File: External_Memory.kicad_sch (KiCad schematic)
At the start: 2 parts, among them U5 GD25D10CT

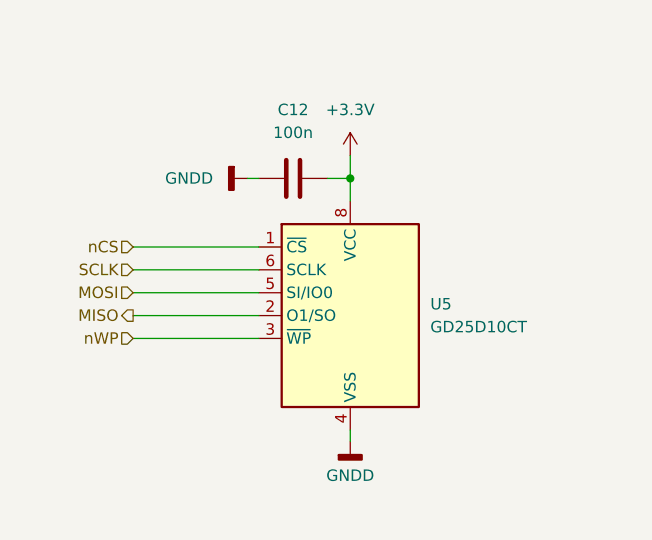
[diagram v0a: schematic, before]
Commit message: wip
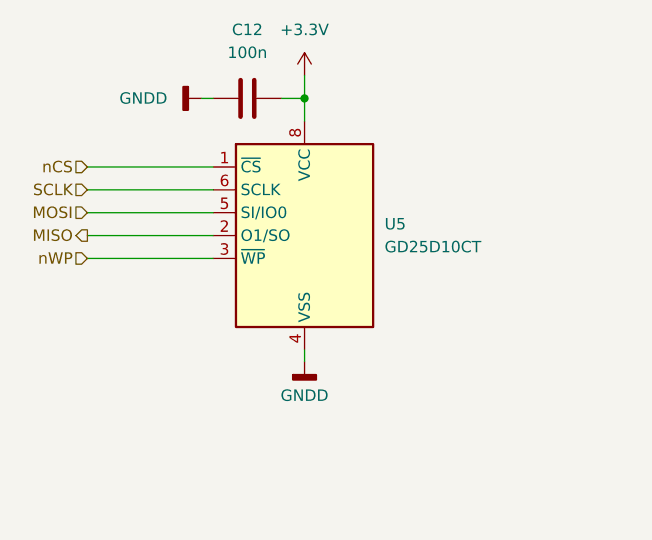
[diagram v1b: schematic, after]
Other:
- moved on the sheet: C12, U5
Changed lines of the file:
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@@
 	(paper "A5")
 	(junction
-		(at 80.01 40.64)
+		(at 74.93 31.75)
 		(diameter 0)
 		(color 0 0 0 0)
@@
 	(wire
 		(pts
-			(xy 80.01 68.58) (xy 80.01 69.85)
-		)
-		(stroke
-			(width 0)
-			(type default)
-		)
-	)
-	(wire
-		(pts
-			(xy 55.88 53.34) (xy 69.85 53.34)
-		)
-		(stroke
-			(width 0)
-			(type default)
-		)
-	)
-	(wire
-		(pts
-			(xy 55.88 50.8) (xy 69.85 50.8)
-		)
-		(stroke
-			(width 0)
-			(type default)
-		)
-	)
-	(wire
-		(pts
-			(xy 55.88 58.42) (xy 69.85 58.42)
-		)
-		(stroke
-			(width 0)
-			(type default)
-		)
-	)
-	(wire
-		(pts
-			(xy 68.58 40.64) (xy 69.85 40.64)
-		)
-		(stroke
-			(width 0)
-			(type default)
-		)
-	)
-	(wire
-		(pts
-			(xy 55.88 55.88) (xy 69.85 55.88)
-		)
-		(stroke
-			(width 0)
-			(type default)
-		)
-	)
-	(wire
-		(pts
-			(xy 80.01 38.1) (xy 80.01 40.64)
-		)
-		(stroke
-			(width 0)
-			(type default)
-		)
-	)
-	(wire
-		(pts
-			(xy 55.88 48.26) (xy 69.85 48.26)
-		)
-		(stroke
-			(width 0)
-			(type default)
-		)
-	)
-	(wire
-		(pts
-			(xy 77.47 40.64) (xy 80.01 40.64)
-		)
-		(stroke
-			(width 0)
-			(type default)
-		)
-	)
-	(wire
-		(pts
-			(xy 80.01 40.64) (xy 80.01 43.18)
+			(xy 74.93 59.69) (xy 74.93 60.96)
+		)
+		(stroke
+			(width 0)
+			(type default)
+		)
+	)
+	(wire
+		(pts
+			(xy 50.8 44.45) (xy 64.77 44.45)
+		)
+		(stroke
+			(width 0)
+			(type default)
+		)
+	)
+	(wire
+		(pts
+			(xy 50.8 41.91) (xy 64.77 41.91)
+		)
+		(stroke
+			(width 0)
+			(type default)
+		)
+	)
+	(wire
+		(pts
+			(xy 50.8 49.53) (xy 64.77 49.53)
+		)
+		(stroke
+			(width 0)
+			(type default)
+		)
+	)
+	(wire
+		(pts
+			(xy 63.5 31.75) (xy 64.77 31.75)
+		)
+		(stroke
+			(width 0)
+			(type default)
+		)
+	)
+	(wire
+		(pts
+			(xy 50.8 46.99) (xy 64.77 46.99)
+		)
+		(stroke
+			(width 0)
+			(type default)
+		)
+	)
+	(wire
+		(pts
+			(xy 74.93 29.21) (xy 74.93 31.75)
+		)
+		(stroke
+			(width 0)
+			(type default)
+		)
+	)
+	(wire
+		(pts
+			(xy 50.8 39.37) (xy 64.77 39.37)
+		)
+		(stroke
+			(width 0)
+			(type default)
+		)
+	)
+	(wire
+		(pts
+			(xy 72.39 31.75) (xy 74.93 31.75)
+		)
+		(stroke
+			(width 0)
+			(type default)
+		)
+	)
+	(wire
+		(pts
+			(xy 74.93 31.75) (xy 74.93 34.29)
 		)
 		(stroke
@@
 	(hierarchical_label "nCS"
 		(shape input)
-		(at 55.88 48.26 180)
+		(at 50.8 39.37 180)
 		(effects
 			(font
@@
 	(hierarchical_label "SCLK"
 		(shape input)
-		(at 55.88 50.8 180)
+		(at 50.8 41.91 180)
 		(effects
 			(font
@@
 	(hierarchical_label "nWP"
 		(shape input)
-		(at 55.88 58.42 180)
+		(at 50.8 49.53 180)
 		(effects
 			(font
@@
 	(hierarchical_label "MOSI"
 		(shape input)
-		(at 55.88 53.34 180)
+		(at 50.8 44.45 180)
 		(effects
 			(font
@@
 	(hierarchical_label "MISO"
 		(shape output)
-		(at 55.88 55.88 180)
+		(at 50.8 46.99 180)
 		(effects
 			(font
@@
 	(symbol
 		(lib_id "power:GNDD")
-		(at 68.58 40.64 270)
+		(at 63.5 31.75 270)
 		(unit 1)
 		(exclude_from_sim no)
@@
 		(fields_autoplaced yes)
 		(property "Reference" "#PWR032"
-			(at 62.23 40.64 0)
+			(at 57.15 31.75 0)
 			(effects
 				(font
@@
 		)
 		(property "Value" "GNDD"
-			(at 64.77 40.6399 90)
+			(at 59.69 31.7499 90)
 			(effects
 				(font
@@
 		)
 		(property "Footprint" ""
-			(at 68.58 40.64 0)
+			(at 63.5 31.75 0)
 			(effects
 				(font
@@
 		)
 		(property "Datasheet" ""
-			(at 68.58 40.64 0)
+			(at 63.5 31.75 0)
 			(effects
 				(font
@@
 		)
 		(property "Description" "Power symbol creates a global label with name \"GNDD\" , digital ground"
-			(at 68.58 40.64 0)
+			(at 63.5 31.75 0)
 			(effects
 				(font
@@
 	(symbol
 		(lib_id "Memory_Flash:GD25D10CT")
-		(at 80.01 55.88 0)
+		(at 74.93 46.99 0)
 		(unit 1)
 		(exclude_from_sim no)
@@
 		(fields_autoplaced yes)
 		(property "Reference" "U5"
-			(at 88.9 54.6099 0)
+			(at 83.82 45.7199 0)
 			(effects
 				(font
@@
 		)
 		(property "Value" "GD25D10CT"
-			(at 88.9 57.1499 0)
+			(at 83.82 48.2599 0)
 			(effects
 				(font
@@
 		)
 		(property "Footprint" "Package_SO:JEITA_SOIC-8_3.9x4.9mm_P1.27mm"
-			(at 80.01 71.12 0)
+			(at 74.93 62.23 0)
 			(effects
 				(font
@@
 		)
 		(property "Datasheet" "http://www.elm-tech.com/en/products/spi-flash-memory/gd25d10/gd25d10.pdf"
-			(at 80.01 55.88 0)
+			(at 74.93 46.99 0)
 			(effects
 				(font
@@
 		)
 		(property "Description" "1Mbit, 3.0V Standard and Dual Serial Flash, JEITA SOIC-8 (SOP-8)"
-			(at 80.01 55.88 0)
+			(at 74.93 46.99 0)
 			(effects
 				(font
@@
 	(symbol
 		(lib_id "power:GNDD")
-		(at 80.01 69.85 0)
+		(at 74.93 60.96 0)
 		(unit 1)
 		(exclude_from_sim no)
@@
 		(fields_autoplaced yes)
 		(property "Reference" "#PWR031"
-			(at 80.01 76.2 0)
+			(at 74.93 67.31 0)
 			(effects
 				(font
@@
 		)
 		(property "Value" "GNDD"
-			(at 80.01 73.66 0)
+			(at 74.93 64.77 0)
 			(effects
 				(font
@@
 		)
 		(property "Footprint" ""
-			(at 80.01 69.85 0)
+			(at 74.93 60.96 0)
 			(effects
 				(font
@@
 		)
 		(property "Datasheet" ""
-			(at 80.01 69.85 0)
+			(at 74.93 60.96 0)
 			(effects
 				(font
@@
 		)
 		(property "Description" "Power symbol creates a global label with name \"GNDD\" , digital ground"
-			(at 80.01 69.85 0)
+			(at 74.93 60.96 0)
 			(effects
 				(font
@@
 	(symbol
 		(lib_id "Device:C")
-		(at 73.66 40.64 270)
+		(at 68.58 31.75 270)
 		(unit 1)
 		(exclude_from_sim no)
@@
 		(fields_autoplaced yes)
 		(property "Reference" "C12"
-			(at 73.66 33.02 90)
+			(at 68.58 24.13 90)
 			(effects
 				(font
@@
 		)
 		(property "Value" "100n"
-			(at 73.66 35.56 90)
+			(at 68.58 26.67 90)
 			(effects
 				(font
@@
 		)
 		(property "Footprint" "Capacitor_SMD:C_0805_2012Metric_Pad1.18x1.45mm_HandSolder"
-			(at 69.85 41.6052 0)
+			(at 64.77 32.7152 0)
 			(effects
 				(font
@@
 		)
 		(property "Datasheet" "~"
-			(at 73.66 40.64 0)
+			(at 68.58 31.75 0)
 			(effects
 				(font
@@
 		)
 		(property "Description" "Unpolarized capacitor"
-			(at 73.66 40.64 0)
+			(at 68.58 31.75 0)
 			(effects
 				(font
@@
 	(symbol
 		(lib_id "power:+3.3V")
-		(at 80.01 38.1 0)
+		(at 74.93 29.21 0)
 		(unit 1)
 		(exclude_from_sim no)
@@
 		(fields_autoplaced yes)
 		(property "Reference" "#PWR030"
-			(at 80.01 41.91 0)
+			(at 74.93 33.02 0)
 			(effects
 				(font
@@
 		)
 		(property "Value" "+3.3V"
-			(at 80.01 33.02 0)
+			(at 74.93 24.13 0)
 			(effects
 				(font
@@
 		)
 		(property "Footprint" ""
-			(at 80.01 38.1 0)
+			(at 74.93 29.21 0)
 			(effects
 				(font
@@
 		)
 		(property "Datasheet" ""
-			(at 80.01 38.1 0)
+			(at 74.93 29.21 0)
 			(effects
 				(font
@@
 		)
 		(property "Description" "Power symbol creates a global label with name \"+3.3V\""
-			(at 80.01 38.1 0)
-			(effects
-				(font
+			(at 74.93 29.21 0)
+			(effects
+				(font

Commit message: wip
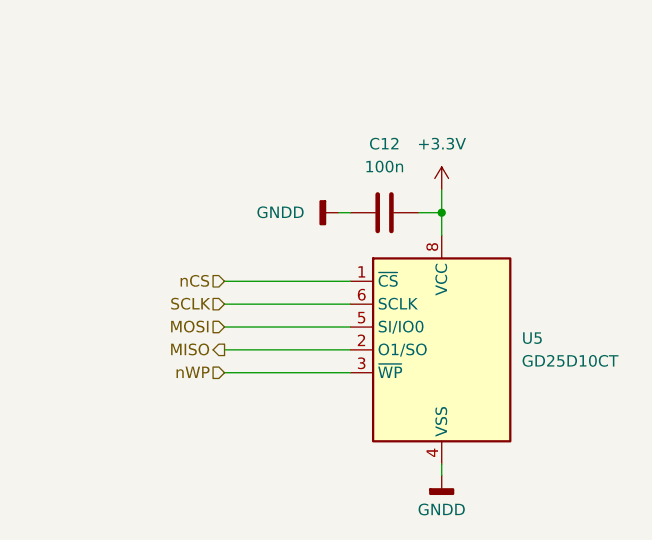
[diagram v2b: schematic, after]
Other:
- moved on the sheet: C12, U5
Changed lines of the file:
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@@
 	(paper "A5")
 	(junction
-		(at 74.93 31.75)
+		(at 90.17 44.45)
 		(diameter 0)
 		(color 0 0 0 0)
@@
 	(wire
 		(pts
-			(xy 74.93 59.69) (xy 74.93 60.96)
-		)
-		(stroke
-			(width 0)
-			(type default)
-		)
-	)
-	(wire
-		(pts
-			(xy 50.8 44.45) (xy 64.77 44.45)
-		)
-		(stroke
-			(width 0)
-			(type default)
-		)
-	)
-	(wire
-		(pts
-			(xy 50.8 41.91) (xy 64.77 41.91)
-		)
-		(stroke
-			(width 0)
-			(type default)
-		)
-	)
-	(wire
-		(pts
-			(xy 50.8 49.53) (xy 64.77 49.53)
-		)
-		(stroke
-			(width 0)
-			(type default)
-		)
-	)
-	(wire
-		(pts
-			(xy 63.5 31.75) (xy 64.77 31.75)
-		)
-		(stroke
-			(width 0)
-			(type default)
-		)
-	)
-	(wire
-		(pts
-			(xy 50.8 46.99) (xy 64.77 46.99)
-		)
-		(stroke
-			(width 0)
-			(type default)
-		)
-	)
-	(wire
-		(pts
-			(xy 74.93 29.21) (xy 74.93 31.75)
-		)
-		(stroke
-			(width 0)
-			(type default)
-		)
-	)
-	(wire
-		(pts
-			(xy 50.8 39.37) (xy 64.77 39.37)
-		)
-		(stroke
-			(width 0)
-			(type default)
-		)
-	)
-	(wire
-		(pts
-			(xy 72.39 31.75) (xy 74.93 31.75)
-		)
-		(stroke
-			(width 0)
-			(type default)
-		)
-	)
-	(wire
-		(pts
-			(xy 74.93 31.75) (xy 74.93 34.29)
+			(xy 90.17 72.39) (xy 90.17 73.66)
+		)
+		(stroke
+			(width 0)
+			(type default)
+		)
+	)
+	(wire
+		(pts
+			(xy 66.04 57.15) (xy 80.01 57.15)
+		)
+		(stroke
+			(width 0)
+			(type default)
+		)
+	)
+	(wire
+		(pts
+			(xy 66.04 54.61) (xy 80.01 54.61)
+		)
+		(stroke
+			(width 0)
+			(type default)
+		)
+	)
+	(wire
+		(pts
+			(xy 66.04 62.23) (xy 80.01 62.23)
+		)
+		(stroke
+			(width 0)
+			(type default)
+		)
+	)
+	(wire
+		(pts
+			(xy 78.74 44.45) (xy 80.01 44.45)
+		)
+		(stroke
+			(width 0)
+			(type default)
+		)
+	)
+	(wire
+		(pts
+			(xy 66.04 59.69) (xy 80.01 59.69)
+		)
+		(stroke
+			(width 0)
+			(type default)
+		)
+	)
+	(wire
+		(pts
+			(xy 90.17 41.91) (xy 90.17 44.45)
+		)
+		(stroke
+			(width 0)
+			(type default)
+		)
+	)
+	(wire
+		(pts
+			(xy 66.04 52.07) (xy 80.01 52.07)
+		)
+		(stroke
+			(width 0)
+			(type default)
+		)
+	)
+	(wire
+		(pts
+			(xy 87.63 44.45) (xy 90.17 44.45)
+		)
+		(stroke
+			(width 0)
+			(type default)
+		)
+	)
+	(wire
+		(pts
+			(xy 90.17 44.45) (xy 90.17 46.99)
 		)
 		(stroke
@@
 	(hierarchical_label "nCS"
 		(shape input)
-		(at 50.8 39.37 180)
+		(at 66.04 52.07 180)
 		(effects
 			(font
@@
 	(hierarchical_label "SCLK"
 		(shape input)
-		(at 50.8 41.91 180)
+		(at 66.04 54.61 180)
 		(effects
 			(font
@@
 	(hierarchical_label "nWP"
 		(shape input)
-		(at 50.8 49.53 180)
+		(at 66.04 62.23 180)
 		(effects
 			(font
@@
 	(hierarchical_label "MOSI"
 		(shape input)
-		(at 50.8 44.45 180)
+		(at 66.04 57.15 180)
 		(effects
 			(font
@@
 	(hierarchical_label "MISO"
 		(shape output)
-		(at 50.8 46.99 180)
+		(at 66.04 59.69 180)
 		(effects
 			(font
@@
 	(symbol
 		(lib_id "power:GNDD")
-		(at 63.5 31.75 270)
+		(at 78.74 44.45 270)
 		(unit 1)
 		(exclude_from_sim no)
@@
 		(fields_autoplaced yes)
 		(property "Reference" "#PWR032"
-			(at 57.15 31.75 0)
+			(at 72.39 44.45 0)
 			(effects
 				(font
@@
 		)
 		(property "Value" "GNDD"
-			(at 59.69 31.7499 90)
+			(at 74.93 44.4499 90)
 			(effects
 				(font
@@
 		)
 		(property "Footprint" ""
-			(at 63.5 31.75 0)
+			(at 78.74 44.45 0)
 			(effects
 				(font
@@
 		)
 		(property "Datasheet" ""
-			(at 63.5 31.75 0)
+			(at 78.74 44.45 0)
 			(effects
 				(font
@@
 		)
 		(property "Description" "Power symbol creates a global label with name \"GNDD\" , digital ground"
-			(at 63.5 31.75 0)
+			(at 78.74 44.45 0)
 			(effects
 				(font
@@
 	(symbol
 		(lib_id "Memory_Flash:GD25D10CT")
-		(at 74.93 46.99 0)
+		(at 90.17 59.69 0)
 		(unit 1)
 		(exclude_from_sim no)
@@
 		(fields_autoplaced yes)
 		(property "Reference" "U5"
-			(at 83.82 45.7199 0)
+			(at 99.06 58.4199 0)
 			(effects
 				(font
@@
 		)
 		(property "Value" "GD25D10CT"
-			(at 83.82 48.2599 0)
+			(at 99.06 60.9599 0)
 			(effects
 				(font
@@
 		)
 		(property "Footprint" "Package_SO:JEITA_SOIC-8_3.9x4.9mm_P1.27mm"
-			(at 74.93 62.23 0)
+			(at 90.17 74.93 0)
 			(effects
 				(font
@@
 		)
 		(property "Datasheet" "http://www.elm-tech.com/en/products/spi-flash-memory/gd25d10/gd25d10.pdf"
-			(at 74.93 46.99 0)
+			(at 90.17 59.69 0)
 			(effects
 				(font
@@
 		)
 		(property "Description" "1Mbit, 3.0V Standard and Dual Serial Flash, JEITA SOIC-8 (SOP-8)"
-			(at 74.93 46.99 0)
+			(at 90.17 59.69 0)
 			(effects
 				(font
@@
 	(symbol
 		(lib_id "power:GNDD")
-		(at 74.93 60.96 0)
+		(at 90.17 73.66 0)
 		(unit 1)
 		(exclude_from_sim no)
@@
 		(fields_autoplaced yes)
 		(property "Reference" "#PWR031"
-			(at 74.93 67.31 0)
+			(at 90.17 80.01 0)
 			(effects
 				(font
@@
 		)
 		(property "Value" "GNDD"
-			(at 74.93 64.77 0)
+			(at 90.17 77.47 0)
 			(effects
 				(font
@@
 		)
 		(property "Footprint" ""
-			(at 74.93 60.96 0)
+			(at 90.17 73.66 0)
 			(effects
 				(font
@@
 		)
 		(property "Datasheet" ""
-			(at 74.93 60.96 0)
+			(at 90.17 73.66 0)
 			(effects
 				(font
@@
 		)
 		(property "Description" "Power symbol creates a global label with name \"GNDD\" , digital ground"
-			(at 74.93 60.96 0)
+			(at 90.17 73.66 0)
 			(effects
 				(font
@@
 	(symbol
 		(lib_id "Device:C")
-		(at 68.58 31.75 270)
+		(at 83.82 44.45 270)
 		(unit 1)
 		(exclude_from_sim no)
@@
 		(fields_autoplaced yes)
 		(property "Reference" "C12"
-			(at 68.58 24.13 90)
+			(at 83.82 36.83 90)
 			(effects
 				(font
@@
 		)
 		(property "Value" "100n"
-			(at 68.58 26.67 90)
+			(at 83.82 39.37 90)
 			(effects
 				(font
@@
 		)
 		(property "Footprint" "Capacitor_SMD:C_0805_2012Metric_Pad1.18x1.45mm_HandSolder"
-			(at 64.77 32.7152 0)
+			(at 80.01 45.4152 0)
 			(effects
 				(font
@@
 		)
 		(property "Datasheet" "~"
-			(at 68.58 31.75 0)
+			(at 83.82 44.45 0)
 			(effects
 				(font
@@
 		)
 		(property "Description" "Unpolarized capacitor"
-			(at 68.58 31.75 0)
+			(at 83.82 44.45 0)
 			(effects
 				(font
@@
 	(symbol
 		(lib_id "power:+3.3V")
-		(at 74.93 29.21 0)
+		(at 90.17 41.91 0)
 		(unit 1)
 		(exclude_from_sim no)
@@
 		(fields_autoplaced yes)
 		(property "Reference" "#PWR030"
-			(at 74.93 33.02 0)
+			(at 90.17 45.72 0)
 			(effects
 				(font
@@
 		)
 		(property "Value" "+3.3V"
-			(at 74.93 24.13 0)
+			(at 90.17 36.83 0)
 			(effects
 				(font
@@
 		)
 		(property "Footprint" ""
-			(at 74.93 29.21 0)
+			(at 90.17 41.91 0)
 			(effects
 				(font
@@
 		)
 		(property "Datasheet" ""
-			(at 74.93 29.21 0)
+			(at 90.17 41.91 0)
 			(effects
 				(font
@@
 		)
 		(property "Description" "Power symbol creates a global label with name \"+3.3V\""
-			(at 74.93 29.21 0)
-			(effects
-				(font
+			(at 90.17 41.91 0)
+			(effects
+				(font
